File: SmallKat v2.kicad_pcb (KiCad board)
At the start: 4 copper layers, 104 x 99 mm, 324 parts, among them IC1 TPS562201DDCR, IC2 TPS40192DRCT, IC4 MAX34409ETE+, IC5 MAX34409ETE+, IC6 MAX34409ETE+, IC7 MAX34409ETE+, J1 Conn_01x03_Male, J10 Conn_01x03_Male, J11 Conn_01x03_Male, J12 Conn_01x03_Male, J13 Conn_01x03_Male, J14 Conn_01x03_Male, J15 Conn_01x03_Male, J16 Conn_01x03_Male, J17 Conn_01x03_Male, J18 Conn_01x02_Male, J19 USB_C_Receptacle, J2 Conn_01x03_Male, J20 USB_C_Receptacle, J21 Conn_01x05_Male, J3 Conn_01x03_Male, J4 Conn_01x03_Male, J5 Conn_01x03_Male, J6 Conn_01x03_Male, J7 Conn_01x03_Male, J8 Conn_01x03_Male, J9 Conn_01x02_Male, Q1 BUK9M120-100EX, Q10 CSD17307Q5A, Q11 CSD17307Q5A, Q12 Si7141DP, Q2 BUK9M120-100EX, Q3 MMBT3904, Q4 MMBT3904, Q5 MMBT3904, Q6 MMBT3904, Q7 2N3905, Q8 BUK9M120-100EX, Q9 BUK9M120-100EX, SW1 SW_SPST, SW2 SW_SPST, SW3 SW_SPST, SW4 SW_SPST, SW5 SW_SPST, U1 BNO055, U10 MIC5365-3.3YC5, U11 FUSB302BMPX, U12 BQ24770, U13 bq76925, U14 PCA9641, U2 LM2840Y, U3 ESP32-WROOM-32, U4 CP2102N-A01-GQFN24, U5 MCP73831-2-OT, U6 STM32L432KBUx, U7 ESP32-WROOM-32, U8 CP2102N-A01-GQFN24, U9 WIICHUCK, Y1 32.768kHz

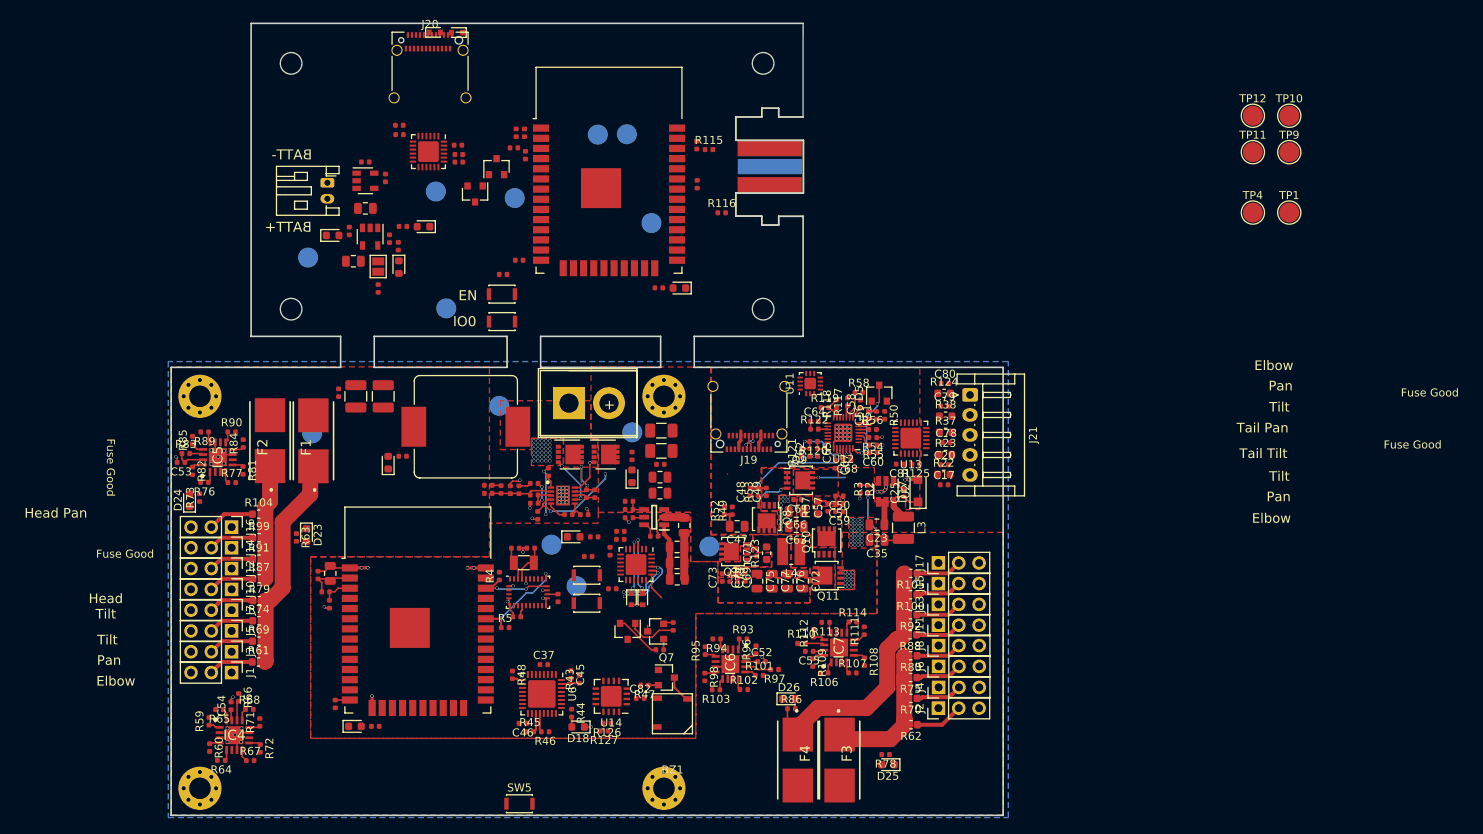
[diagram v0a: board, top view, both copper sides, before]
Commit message: Routing done
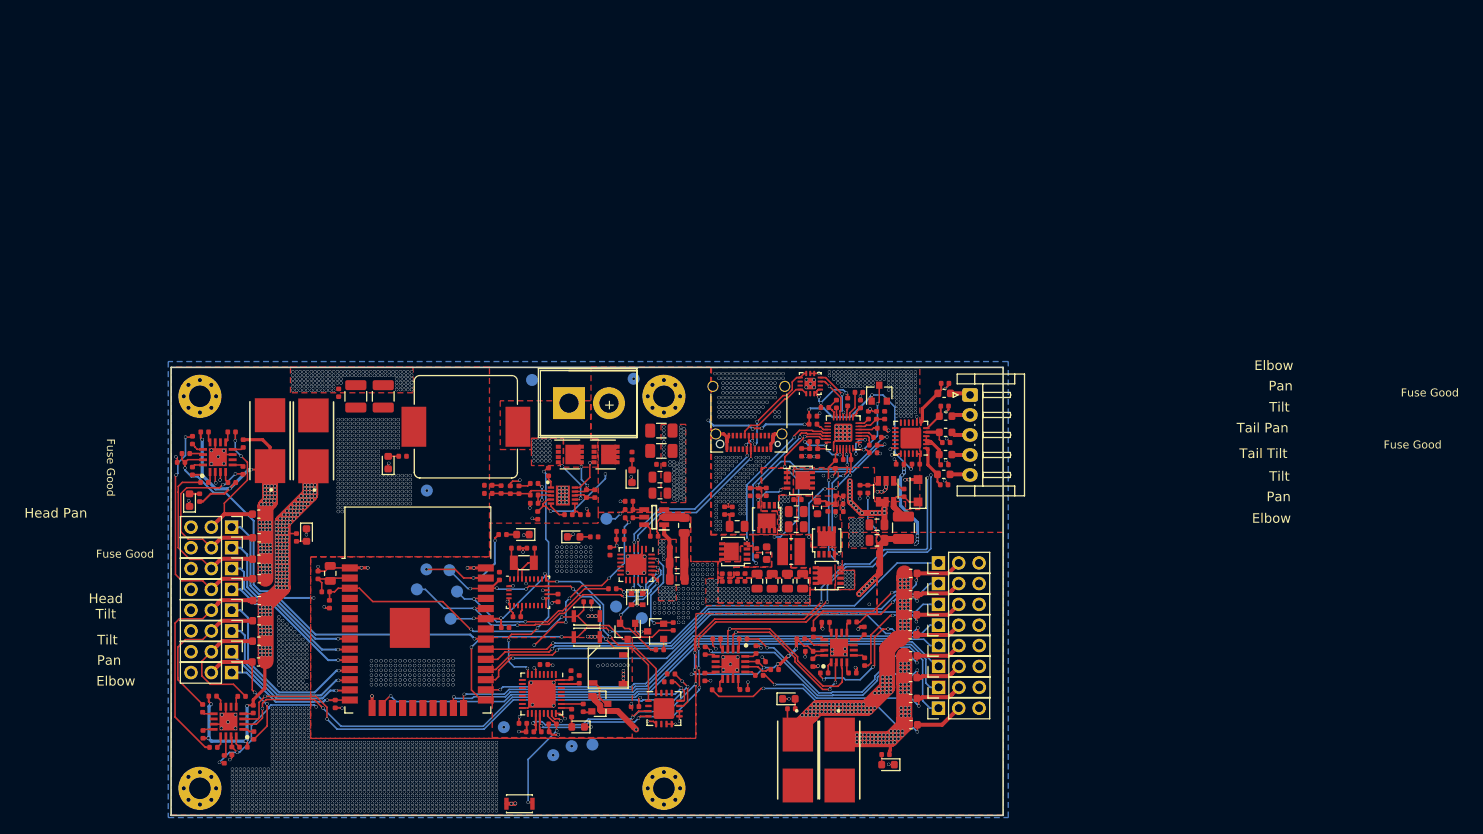
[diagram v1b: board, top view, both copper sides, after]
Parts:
- removed C30, C42: 1uF, Capacitor_SMD:C_0402_1005Metric
- removed C33, C34: 10uF, Capacitor_SMD:C_0805_2012Metric
- removed C36: 22uF, Capacitor_SMD:C_0805_2012Metric
- removed C38, C40, C41, C43, C44: 0.1uF, Capacitor_SMD:C_0402_1005Metric
- removed C39: 4.7uF, Capacitor_SMD:C_0402_1005Metric
- removed D10, D11, D12, D9: LED, LED_SMD:LED_0603_1608Metric
- removed D15, D16: D_TVS, Diode_SMD:D_SOD-523
- removed H5, H6, H7, H8: MountingHole, MountingHole:MountingHole_2.7mm_M2.5
- removed J18: Conn_01x02_Male, Connector_JST:JST_PH_S2B-PH-K_1x02_P2.00mm_Horizontal
- removed J20: USB_C_Receptacle, Connector_USB:USB_C_Receptacle_Amphenol_12401610E4-2A_CircularHoles
- removed JP1: Jumper_NO_Small, Jumper:SolderJumper-2_P1.3mm_Open_Pad1.0x1.5mm
- removed Q5, Q6: MMBT3904, Package_TO_SOT_SMD:SOT-23
- removed R115, R116, R29, R30, R32, R36, R40, R41, R42: 10K, Resistor_SMD:R_0402_1005Metric
- removed R28, R31: 330R, Resistor_SMD:R_0402_1005Metric
- removed R33: 2.5K, Resistor_SMD:R_0402_1005Metric
- removed R34, R35, R39: 470R, Resistor_SMD:R_0402_1005Metric
- removed SW3, SW4: SW_SPST, Button_Switch_SMD:SW_SPST_CK_KXT3
- removed TP13, TP14, TP15, TP16, TP17, TP18, TP19, TP4: TestPoint, TestPoint:TestPoint_Pad_D2.5mm
- removed U10: MIC5365-3.3YC5, Package_TO_SOT_SMD:SOT-23-5
- removed U5: MCP73831-2-OT, Package_TO_SOT_SMD:SOT-23-5
- removed U7: ESP32-WROOM-32, RF_Module:ESP32-WROOM-32
- removed U8: CP2102N-A01-GQFN24, Package_DFN_QFN:QFN-24-1EP_4x4mm_P0.5mm_EP2.6x2.6mm
- removed U9: WIICHUCK, WIICHUCK:CHUCK
- added TP20: TestPoint, TestPoint:TestPoint_Pad_D1.5mm, B.Cu at (146.7, 135.3)
- added TP21: TestPoint, TestPoint:TestPoint_Pad_D1.5mm, B.Cu at (149.0, 134.2)
- added TP22: TestPoint, TestPoint:TestPoint_Pad_D1.5mm, B.Cu at (140.6, 131.8)
- added TP23: TestPoint, TestPoint:TestPoint_Pad_D1.5mm, B.Cu at (151.6, 134.0)
- TP1, TP10, TP11, TP12, TP9: footprint TestPoint:TestPoint_Pad_D2.5mm -> TestPoint:TestPoint_Pad_D1.5mm; moved to B.Cu
- TP2, TP3, TP5, TP6, TP7, TP8: footprint TestPoint:TestPoint_Pad_D2.5mm -> TestPoint:TestPoint_Pad_D1.5mm
- moved TP10 124.1 mm to (129.7, 114.6)
- moved TP9 117.6 mm to (134.7, 114.9)
- moved TP1 116.7 mm to (130.9, 112.1)
- moved TP12 100.5 mm to (154.6, 116.8)
- moved TP11 96.1 mm to (157.8, 118.2)
- moved D1 31.9 mm to (142.9, 107.8), turned to 180 degrees
- moved R1 28.8 mm to (140.4, 107.8), turned to 0 degrees
- moved TP8 16.0 mm to (130.9, 102.3)
- moved TP3 16.0 mm to (133.8, 112.2)
- moved TP2 15.6 mm to (133.9, 118.3)
- moved TP5 13.3 mm to (153.4, 105.8)
- moved R127 11.0 mm to (161.4, 125.2), turned to 0 degrees
- moved BZ1 9.84 mm to (153.6, 124.5), turned to 0 degrees
- moved R67 9.32 mm to (104.2, 128.0), turned to 180 degrees
- moved R126 9.22 mm to (161.1, 126.2), turned to 0 degrees
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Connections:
- C35 pad 1: Net-(C35-Pad1) -> +3.3VA
- C37 pad 1: +3V3 -> +3.3VA
- C45 pad 1: +3V3 -> +3.3VA
- C46 pad 1: +3V3 -> +3.3VA
- L3 pad 2: Net-(C35-Pad1) -> +3.3VA
- R1 pad 1: /MainBoard/SERVO8 -> /MainBoard/ESP32Module/IO23
- R101 pad 2: /MainBoard/Servos/S12 -> /MainBoard/Servos/S10
- R103 pad 2: /MainBoard/Servos/S11 -> /MainBoard/Servos/S9
- R112 pad 2: /MainBoard/Servos/S6 -> /MainBoard/Servos/S16
- R3 pad 1: Net-(C35-Pad1) -> +3.3VA
- R43 pad 2: +3V3 -> +3.3VA
- R45 pad 1: +3V3 -> +3.3VA
- R46 pad 1: +3V3 -> +3.3VA
- R48 pad 1: +3V3 -> +3.3VA
- R76 pad 2: /MainBoard/Servos/S5 -> /MainBoard/Servos/S6
- R81 pad 2: /MainBoard/Servos/S6 -> /MainBoard/Servos/S7
- R85 pad 2: /MainBoard/Servos/S8 -> /MainBoard/Servos/S5
- R90 pad 2: /MainBoard/Servos/S7 -> /MainBoard/Servos/S8
- R93 pad 2: /MainBoard/Servos/S9 -> /MainBoard/Servos/S12
- R95 pad 2: /MainBoard/Servos/S10 -> /MainBoard/Servos/S11
- TP1 pad 1: /MainBoard/SERVO8 -> /MainBoard/ESP32Module/IO23
- U14 pad 1: /MainBoard/SAFETYSCL -> /MainBoard/SCL
- U14 pad 16: /MainBoard/SAFETYSDA -> /MainBoard/SDA
- U14 pad 3: /MainBoard/SCL -> /MainBoard/SAFETYSCL
- U14 pad 4: /MainBoard/SDA -> /MainBoard/SAFETYSDA
- U3 pad 37: (no net) -> /MainBoard/ESP32Module/IO23
- U6 pad 1: +3V3 -> +3.3VA
- U6 pad 14: /MainBoard/SafetyMCU/MONITORING -> (no net)
- U6 pad 17: +3V3 -> +3.3VA
- U6 pad 22: (no net) -> /MainBoard/SafetyMCU/SOFTPOWER
- U6 pad 23: (no net) -> Net-(TP20-Pad1)
- U6 pad 24: (no net) -> Net-(TP21-Pad1)
- U6 pad 25: Net-(U6-Pad25) -> /MainBoard/SafetyMCU/MONITORING
- U6 pad 26: (no net) -> /MainBoard/SafetyMCU/BUZZER
- U6 pad 5: +3V3 -> +3.3VA
- U6 pad 6: /MainBoard/6VEN -> /MainBoard/3.3VEN
- U6 pad 7: /MainBoard/3.3VEN -> (no net)
- U6 pad 8: /MainBoard/SafetyMCU/BUZZER -> /MainBoard/6VEN
- U6 pad 9: /MainBoard/SafetyMCU/SOFTPOWER -> (no net)
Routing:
- net /MainBoard/_SCL: track 0.00 -> 131.4 mm, vias 0 -> 6
- net /MainBoard/_SDA: track 0.00 -> 128.6 mm, vias 0 -> 7
- net +3V3: track 19.9 -> 144.0 mm, vias 0 -> 254
- net /MainBoard/SAFETYSCL: track 2.39 -> 103.9 mm, vias 0 -> 9
- net /MainBoard/SAFETYSDA: track 2.37 -> 102.0 mm, vias 0 -> 10
- net /MainBoard/SERVO8: track 0.00 -> 80.0 mm, vias 0 -> 1
- net /MainBoard/Servos/6V4: track 33.2 -> 111.9 mm, vias 0 -> 104
- net /MainBoard/Servos/6V1: track 27.3 -> 104.9 mm, vias 0 -> 164
- net /MainBoard/Servos/6V3: track 17.8 -> 90.1 mm, vias 0 -> 71
- net /MainBoard/SERVO9: track 0.00 -> 69.2 mm, vias 0 -> 1
- net /MainBoard/SERVO10: track 0.00 -> 65.4 mm, vias 0 -> 1
- net /MainBoard/SERVO12: track 0.00 -> 62.2 mm, vias 0 -> 1
- net /MainBoard/SERVO15: track 0.00 -> 61.0 mm, vias 0 -> 1
- net +3.3VA: track 0.00 -> 60.7 mm, vias 0 -> 20
- net /MainBoard/SERVO14: track 0.00 -> 60.5 mm, vias 0 -> 1
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- added copper zone on F.Cu, net +3.3VA
- added copper zone on In1.Cu, net +3.3VA
- added copper zone on F.Cu, net +3V3
- added copper zone on In1.Cu, net +3V3
- added copper zone on In1.Cu, net +6V
- added copper zone on In1.Cu, net VBUS
- removed copper zone on F.Cu, net Net-(U6-Pad25)
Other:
- board size 104 x 99 mm -> 104 x 56 mm
- board text removed: "-"
- board text removed: "3.3v"
- board text removed: "5v"
- board text removed: "6v"
- board text removed: "BATT-"
- board text removed: "DTR"
- board text removed: "EN"
- board text removed: "GND"
- board text removed: "IO0"
- board text removed: "IO2"
- board text removed: "Keion Bisland"
- board text removed: "RTS"
- board text removed: "RX"
- board text removed: "Rev 1.1"
- board text removed: "SCL"
- board text removed: "SDA"
- board text removed: "SmallKat Mother Board"
- board text removed: "SmallKat Remote Controller Board"
- board text removed: "TX"
